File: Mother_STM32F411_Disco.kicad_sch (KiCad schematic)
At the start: 4 parts, among them U1 ESP32-DEVKIT-V1

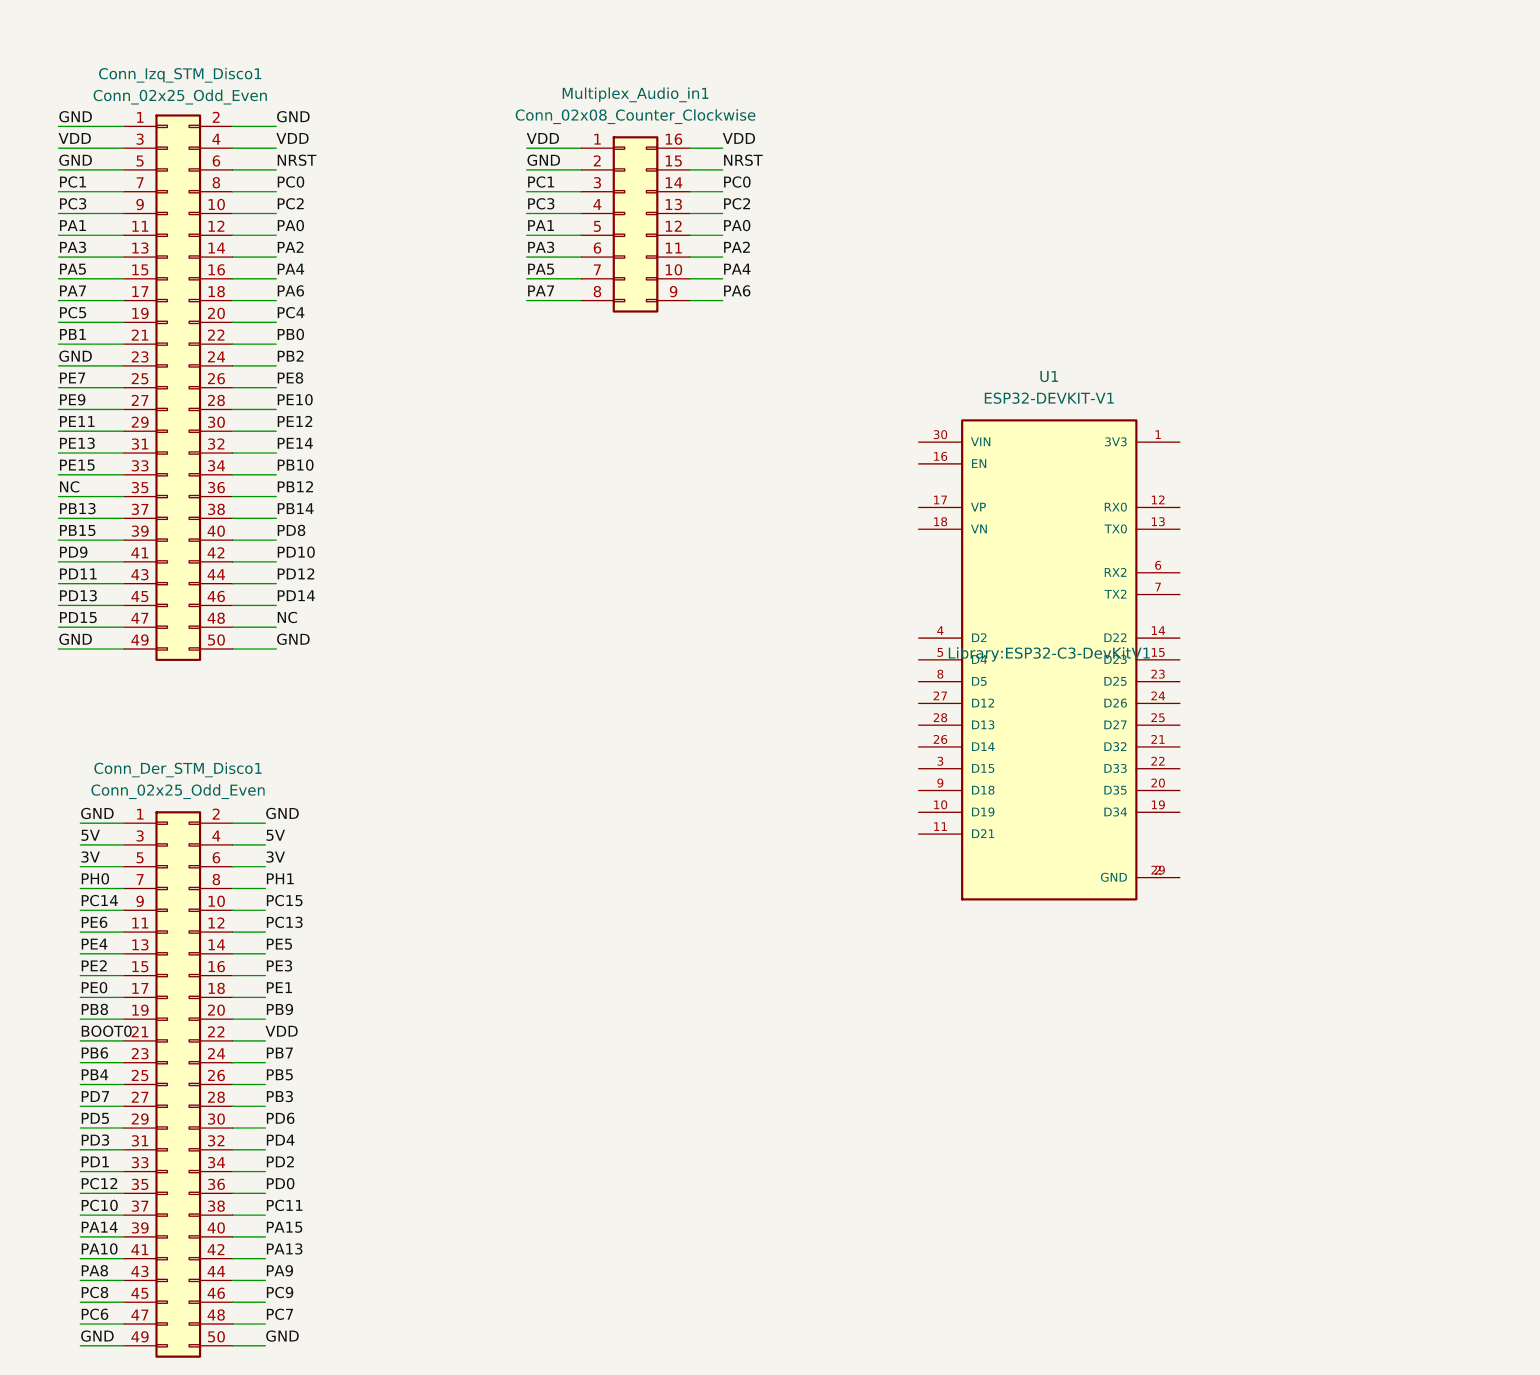
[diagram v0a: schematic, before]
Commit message: .sch mergeado
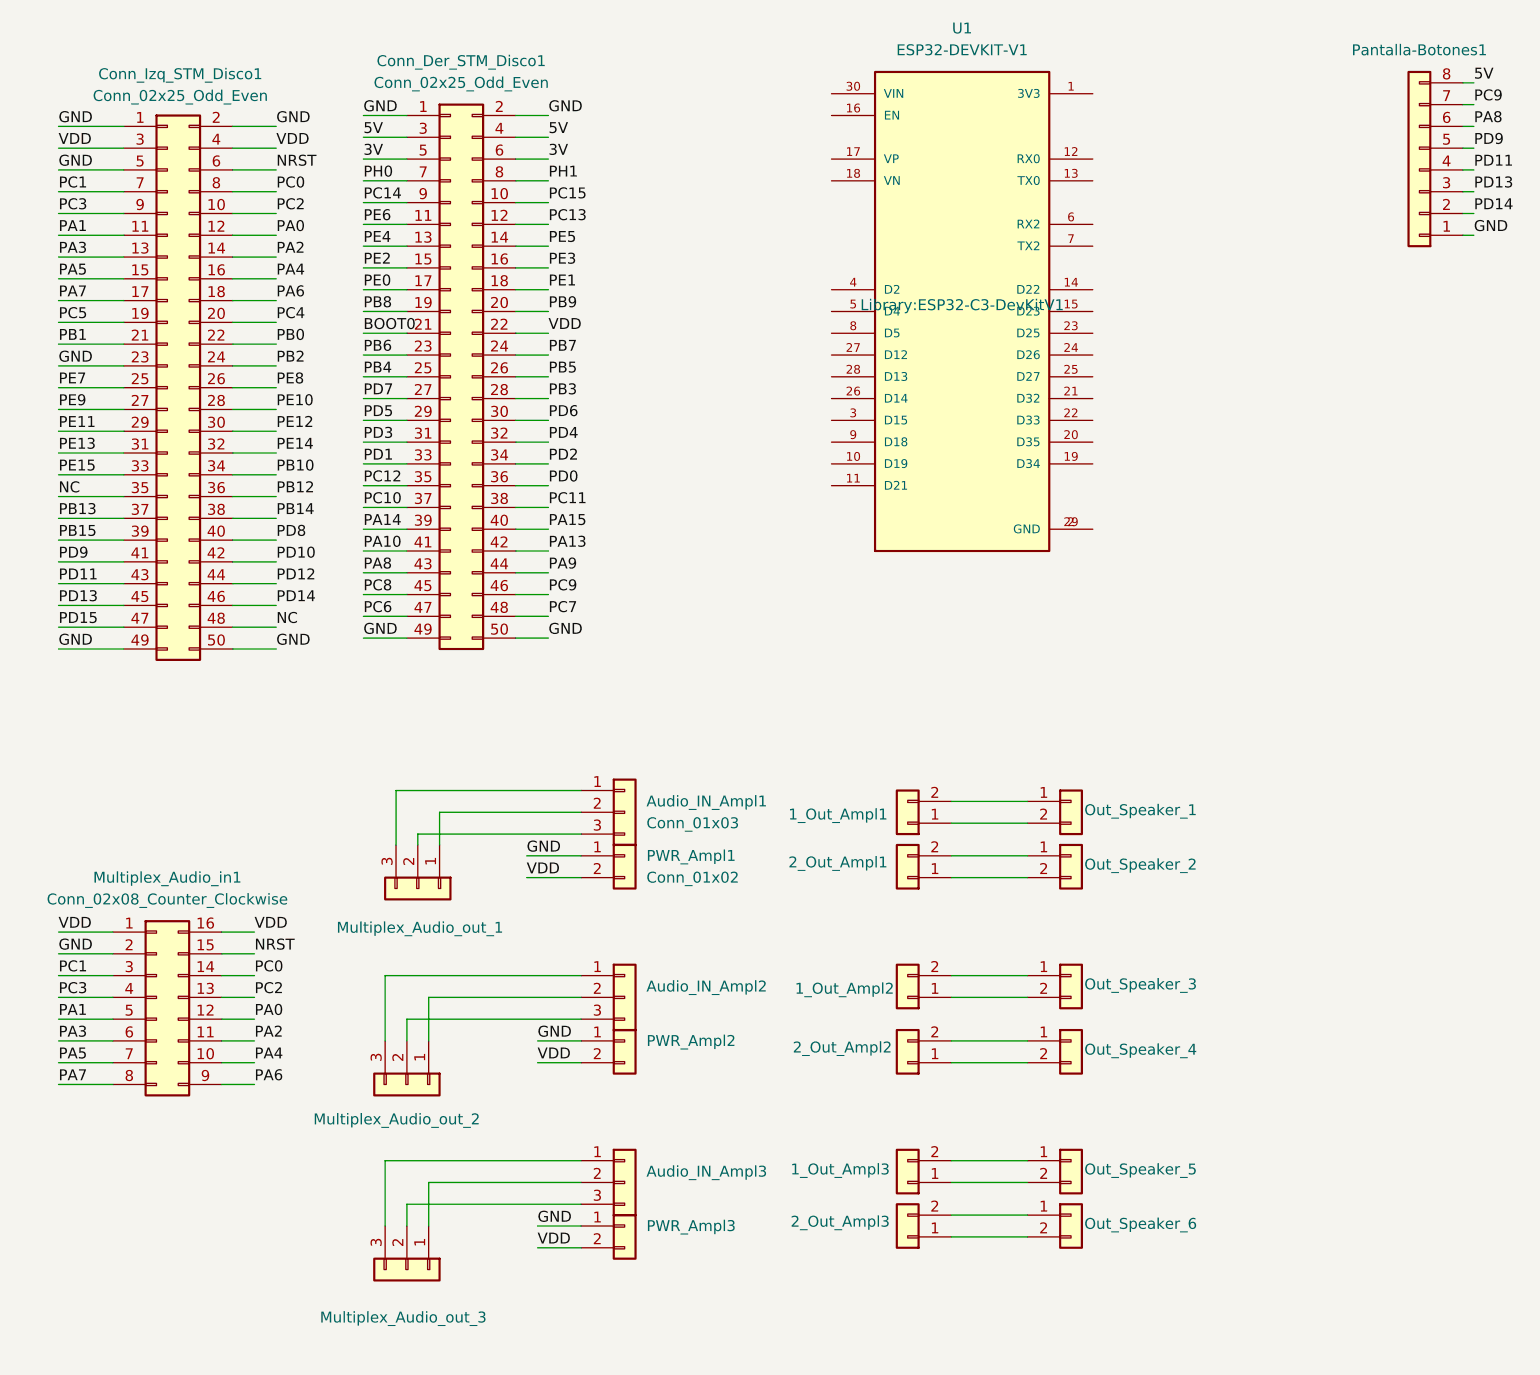
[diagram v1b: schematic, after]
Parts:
- added 1_Out_Ampl1, 1_Out_Ampl2, 1_Out_Ampl3, 2_Out_Ampl1, 2_Out_Ampl2, 2_Out_Ampl3, PWR_Ampl1, PWR_Ampl2, PWR_Ampl3: Conn_01x02, Connector_PinSocket_2.54mm:PinSocket_1x02_P2.54mm_Vertical, symbol Connector_Generic:Conn_01x02
- added Audio_IN_Ampl1, Audio_IN_Ampl2, Audio_IN_Ampl3, Multiplex_Audio_out_1, Multiplex_Audio_out_2, Multiplex_Audio_out_3: Conn_01x03, Connector_PinSocket_2.54mm:PinSocket_1x03_P2.54mm_Vertical, symbol Connector_Generic:Conn_01x03
- added Out_Speaker_1, Out_Speaker_2, Out_Speaker_3, Out_Speaker_4, Out_Speaker_5, Out_Speaker_6: Conn_01x02, Connector_PinHeader_2.54mm:PinHeader_1x02_P2.54mm_Horizontal, symbol Connector_Generic:Conn_01x02
- added Pantalla-Botones1: Conn_01x08, Connector_PinSocket_2.54mm:PinSocket_1x08_P2.54mm_Vertical, symbol Connector_Generic:Conn_01x08
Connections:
- net 5V: now also Pantalla-Botones1.8 (Pin_8)
- net GND: now also PWR_Ampl1.1 (Pin_1), PWR_Ampl2.1 (Pin_1), PWR_Ampl3.1 (Pin_1), Pantalla-Botones1.1 (Pin_1)
- net PA8: now also Pantalla-Botones1.6 (Pin_6)
- net PC9: now also Pantalla-Botones1.7 (Pin_7)
- net PD11: now also Pantalla-Botones1.4 (Pin_4)
- net PD13: now also Pantalla-Botones1.3 (Pin_3)
- net PD14: now also Pantalla-Botones1.2 (Pin_2)
- net PD9: now also Pantalla-Botones1.5 (Pin_5)
- net VDD: now also PWR_Ampl1.2 (Pin_2), PWR_Ampl2.2 (Pin_2), PWR_Ampl3.2 (Pin_2)
- new net: 2_Out_Ampl2.1 (Pin_1), Out_Speaker_4.2 (Pin_2)
- new net: 2_Out_Ampl2.2 (Pin_2), Out_Speaker_4.1 (Pin_1)
- new net: 1_Out_Ampl2.1 (Pin_1), Out_Speaker_3.2 (Pin_2)
- new net: 1_Out_Ampl2.2 (Pin_2), Out_Speaker_3.1 (Pin_1)
- new net: 1_Out_Ampl1.1 (Pin_1), Out_Speaker_1.2 (Pin_2)
- new net: 1_Out_Ampl1.2 (Pin_2), Out_Speaker_1.1 (Pin_1)
- new net: Audio_IN_Ampl3.2 (Pin_2), Multiplex_Audio_out_3.1 (Pin_1)
- new net: Audio_IN_Ampl3.3 (Pin_3), Multiplex_Audio_out_3.2 (Pin_2)
- new net: Audio_IN_Ampl3.1 (Pin_1), Multiplex_Audio_out_3.3 (Pin_3)
- new net: 2_Out_Ampl1.1 (Pin_1), Out_Speaker_2.2 (Pin_2)
- new net: 2_Out_Ampl1.2 (Pin_2), Out_Speaker_2.1 (Pin_1)
- new net: Audio_IN_Ampl2.2 (Pin_2), Multiplex_Audio_out_2.1 (Pin_1)
- new net: Audio_IN_Ampl2.3 (Pin_3), Multiplex_Audio_out_2.2 (Pin_2)
- new net: Audio_IN_Ampl2.1 (Pin_1), Multiplex_Audio_out_2.3 (Pin_3)
- new net: 2_Out_Ampl3.2 (Pin_2), Out_Speaker_6.1 (Pin_1)
- new net: 2_Out_Ampl3.1 (Pin_1), Out_Speaker_6.2 (Pin_2)
- new net: Audio_IN_Ampl1.2 (Pin_2), Multiplex_Audio_out_1.1 (Pin_1)
- new net: Audio_IN_Ampl1.3 (Pin_3), Multiplex_Audio_out_1.2 (Pin_2)
- new net: Audio_IN_Ampl1.1 (Pin_1), Multiplex_Audio_out_1.3 (Pin_3)
- new net: 1_Out_Ampl3.2 (Pin_2), Out_Speaker_5.1 (Pin_1)
- new net: 1_Out_Ampl3.1 (Pin_1), Out_Speaker_5.2 (Pin_2)
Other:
- moved on the sheet: Conn_Der_STM_Disco1, Multiplex_Audio_in1, U1
